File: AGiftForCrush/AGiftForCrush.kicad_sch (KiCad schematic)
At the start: 2 parts

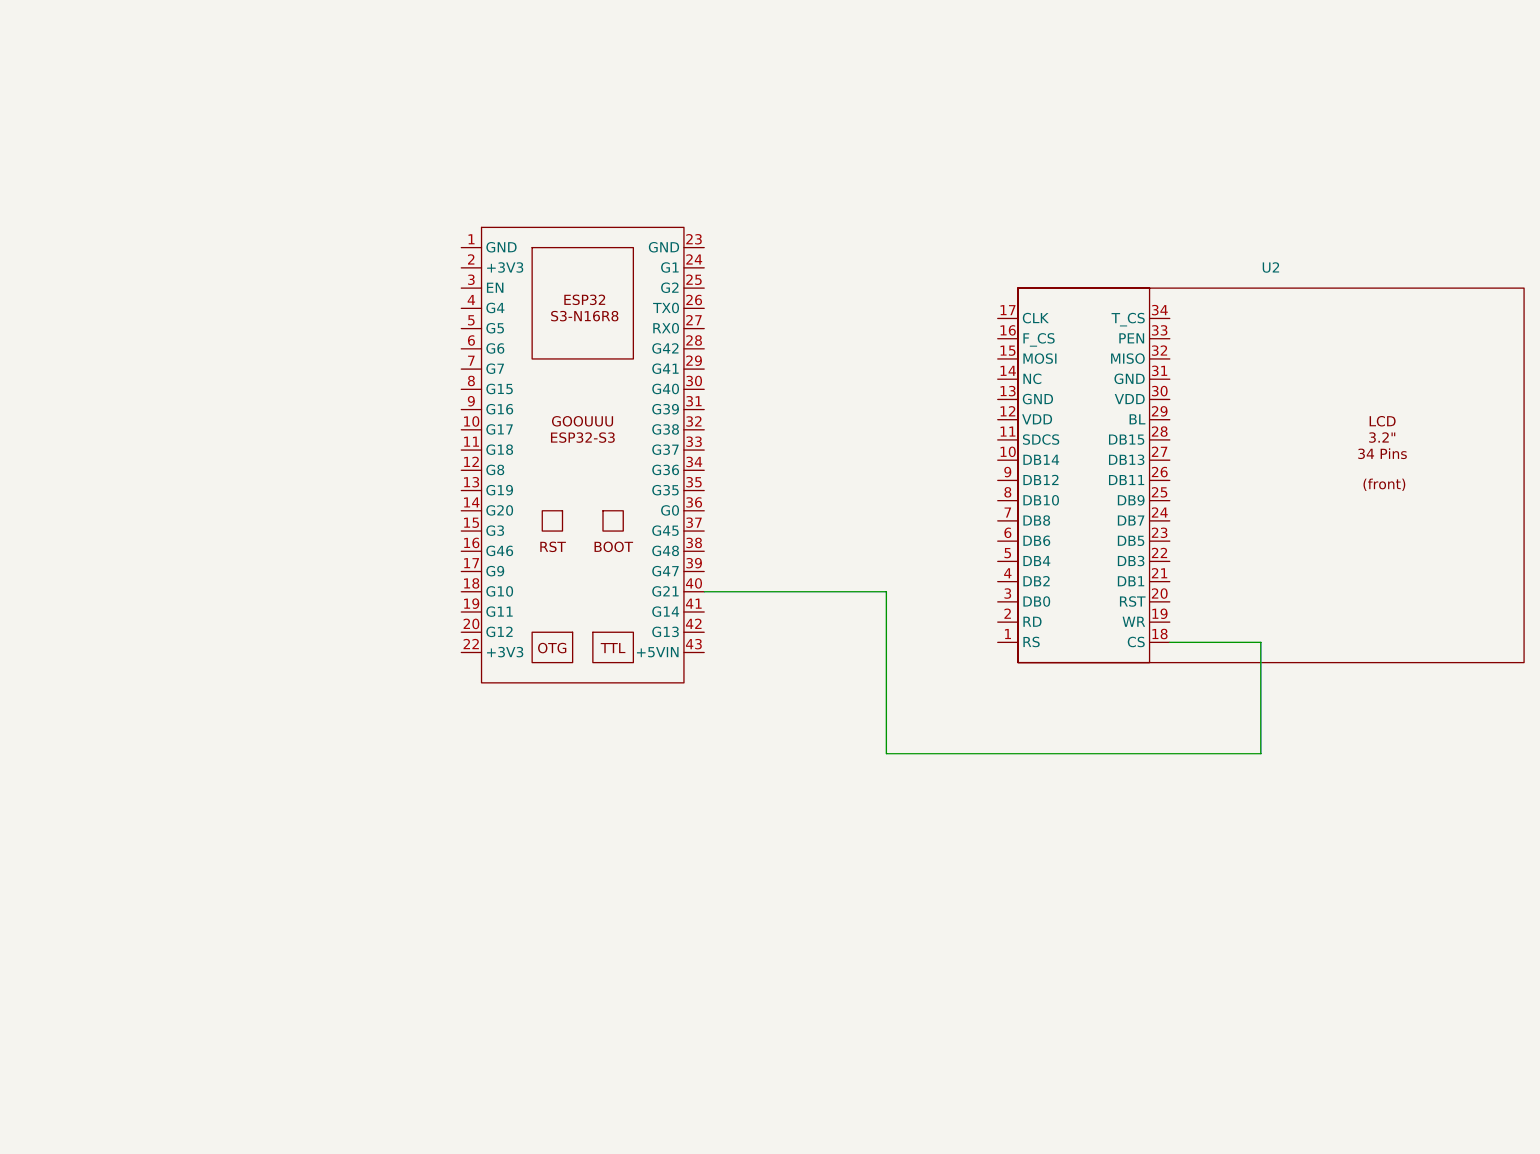
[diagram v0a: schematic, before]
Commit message: Sep 28, Add CodeC
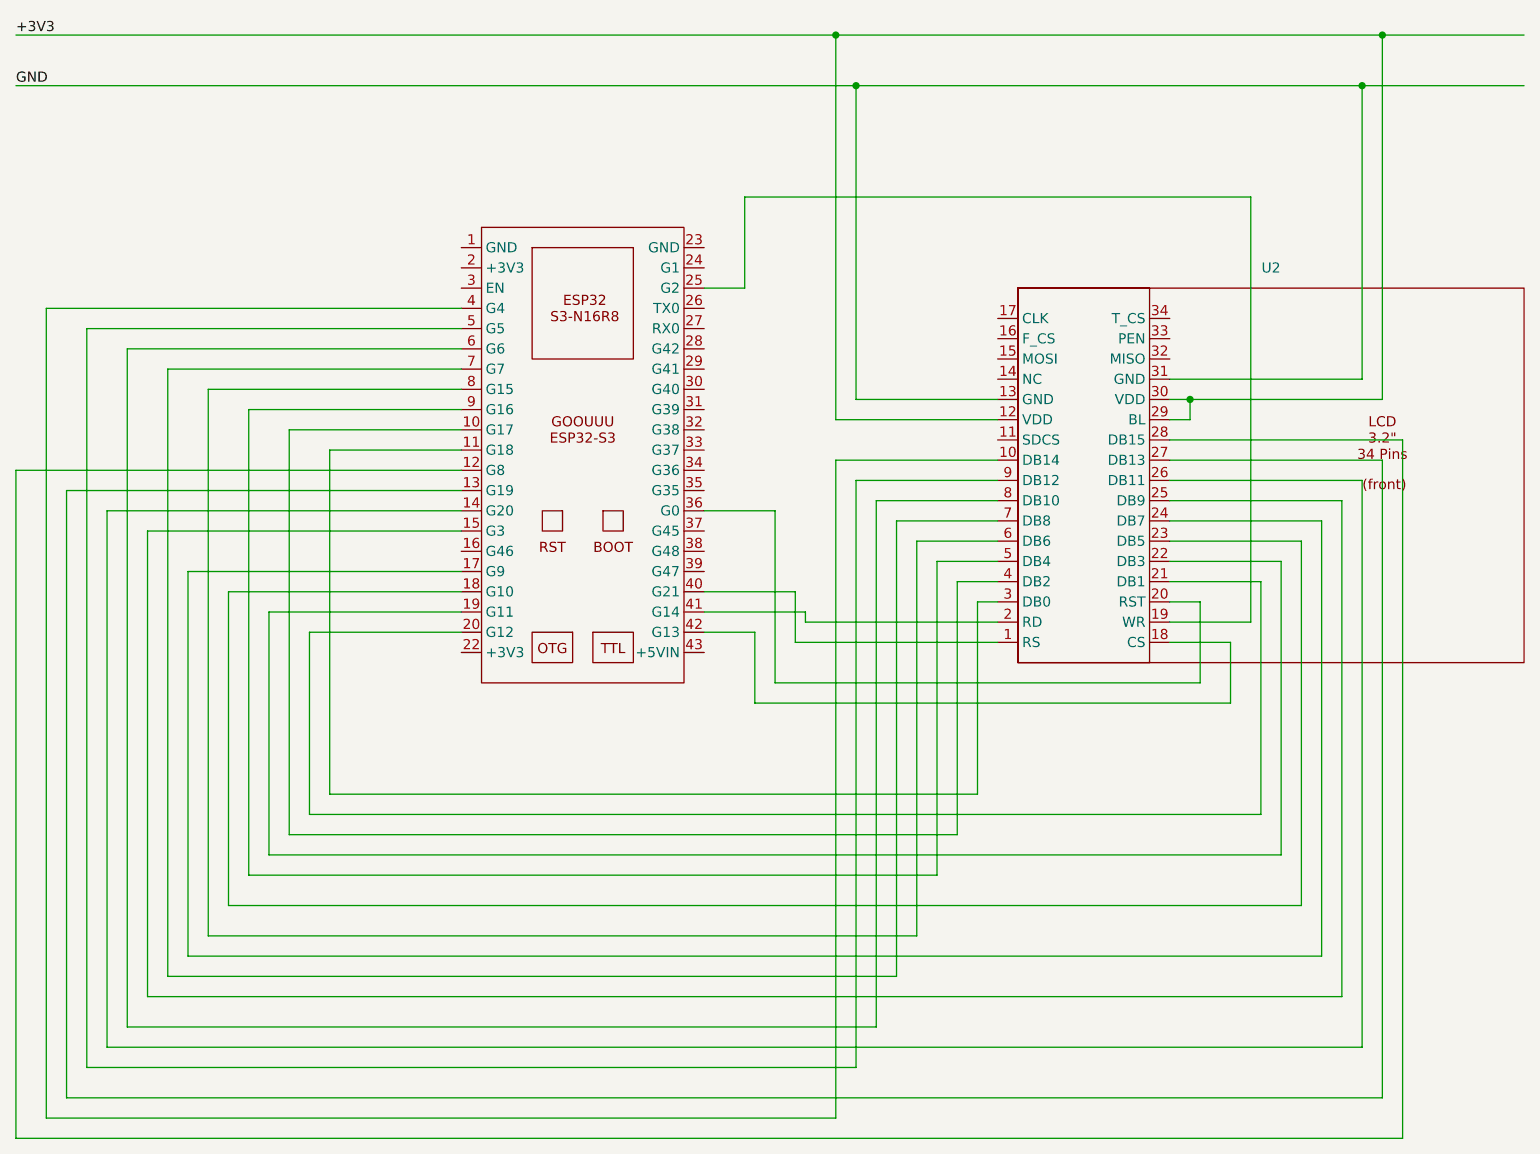
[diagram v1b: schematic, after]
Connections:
- net at U2.1 (RS): now also U1.40 (G21)
- net at U2.10 (DB14): now also U1.4 (G4)
- net +3V3: now reaches U2.12 (VDD)
- net +3V3: now also U2.29 (BL), U2.30 (VDD)
- net GND: now reaches U2.13 (GND)
- net GND: now also U2.31 (GND)
- net at U2.18 (CS): now also U1.42 (G13); no longer U1.40 (G21)
- net at U2.19 (WR): now also U1.25 (G2)
- net at U2.2 (RD): now also U1.41 (G14)
- net at U2.20 (RST): now also U1.36 (G0)
- net at U2.21 (DB1): now also U1.20 (G12)
- net at U2.22 (DB3): now also U1.19 (G11)
- net at U2.23 (DB5): now also U1.18 (G10)
- net at U2.24 (DB7): now also U1.17 (G9)
- net at U2.25 (DB9): now also U1.15 (G3)
- net at U2.26 (DB11): now also U1.14 (G20)
- net at U2.27 (DB13): now also U1.13 (G19)
- net at U2.28 (DB15): now also U1.12 (G8)
- net at U2.3 (DB0): now also U1.11 (G18)
- net at U2.4 (DB2): now also U1.10 (G17)
- net at U2.5 (DB4): now also U1.9 (G16)
- net at U2.6 (DB6): now also U1.8 (G15)
- net at U2.7 (DB8): now also U1.7 (G7)
- net at U2.8 (DB10): now also U1.6 (G6)
- net at U2.9 (DB12): now also U1.5 (G5)
